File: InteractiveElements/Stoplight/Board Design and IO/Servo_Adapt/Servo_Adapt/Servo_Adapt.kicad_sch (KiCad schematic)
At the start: 11 parts, among them J1 RJ45, J2 Conn_01x03_Pin, J3 Conn_01x03_Pin

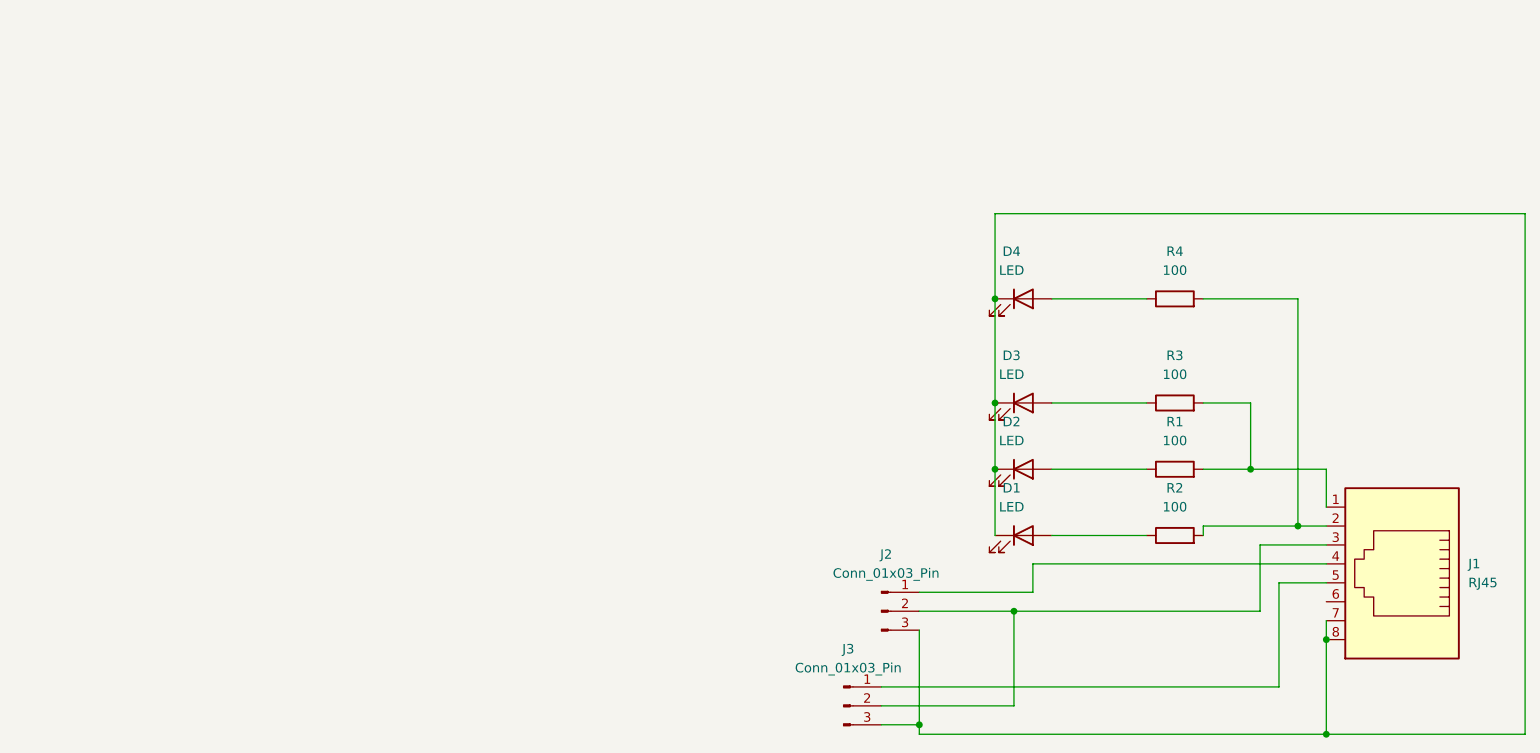
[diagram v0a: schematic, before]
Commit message: file move
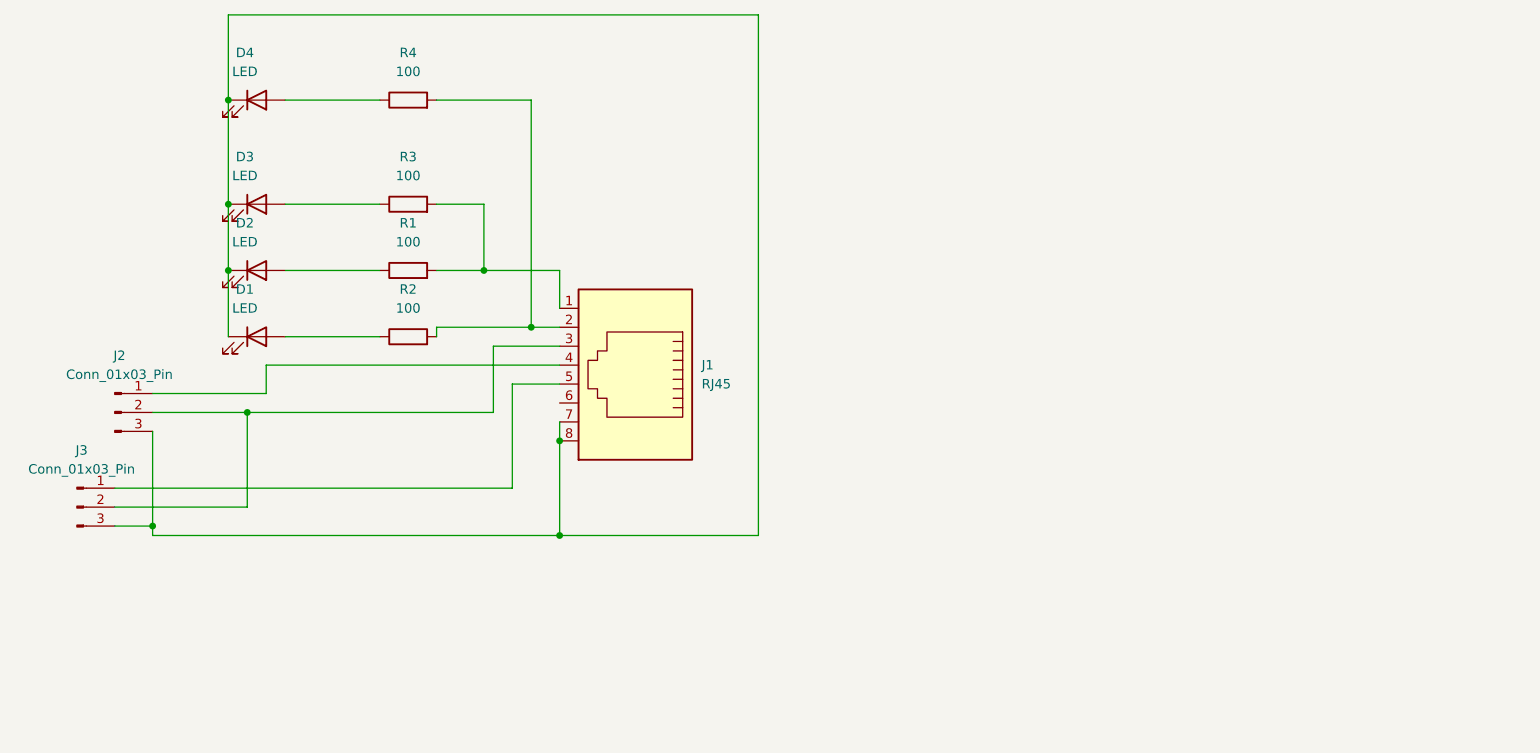
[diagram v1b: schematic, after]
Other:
- title: (none) -> Servo Adapter PCB
- moved on the sheet: D1, D2, D3, D4, J1, J2, J3, R1, R2, R3, R4
